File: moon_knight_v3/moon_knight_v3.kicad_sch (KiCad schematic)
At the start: 12 parts

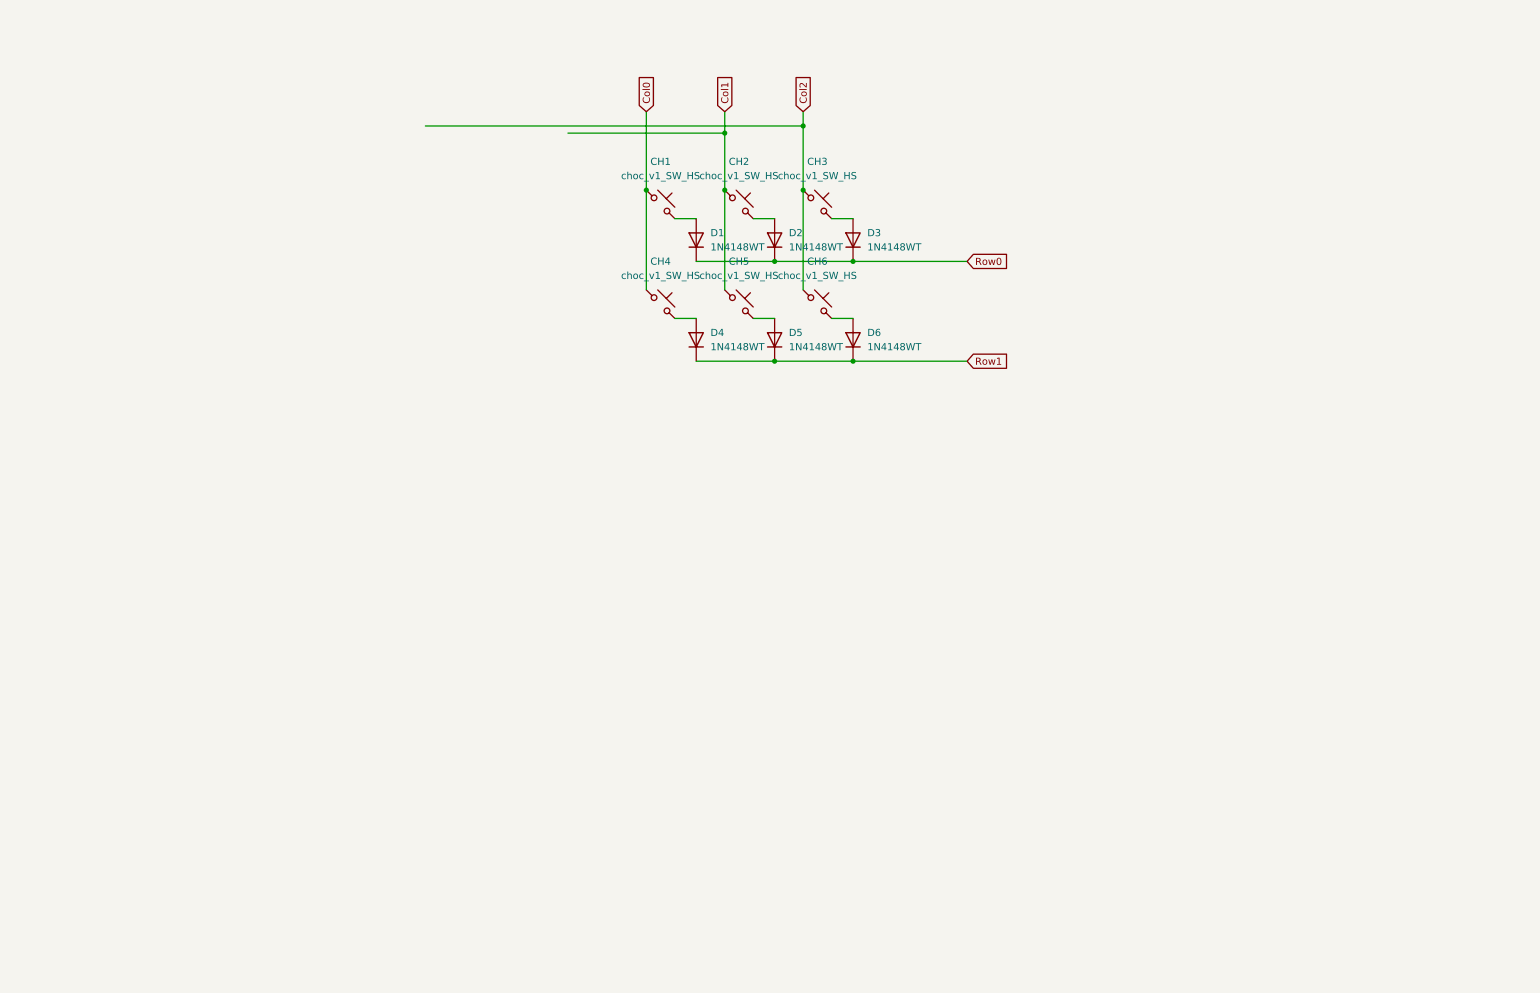
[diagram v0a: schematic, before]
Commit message: some commits
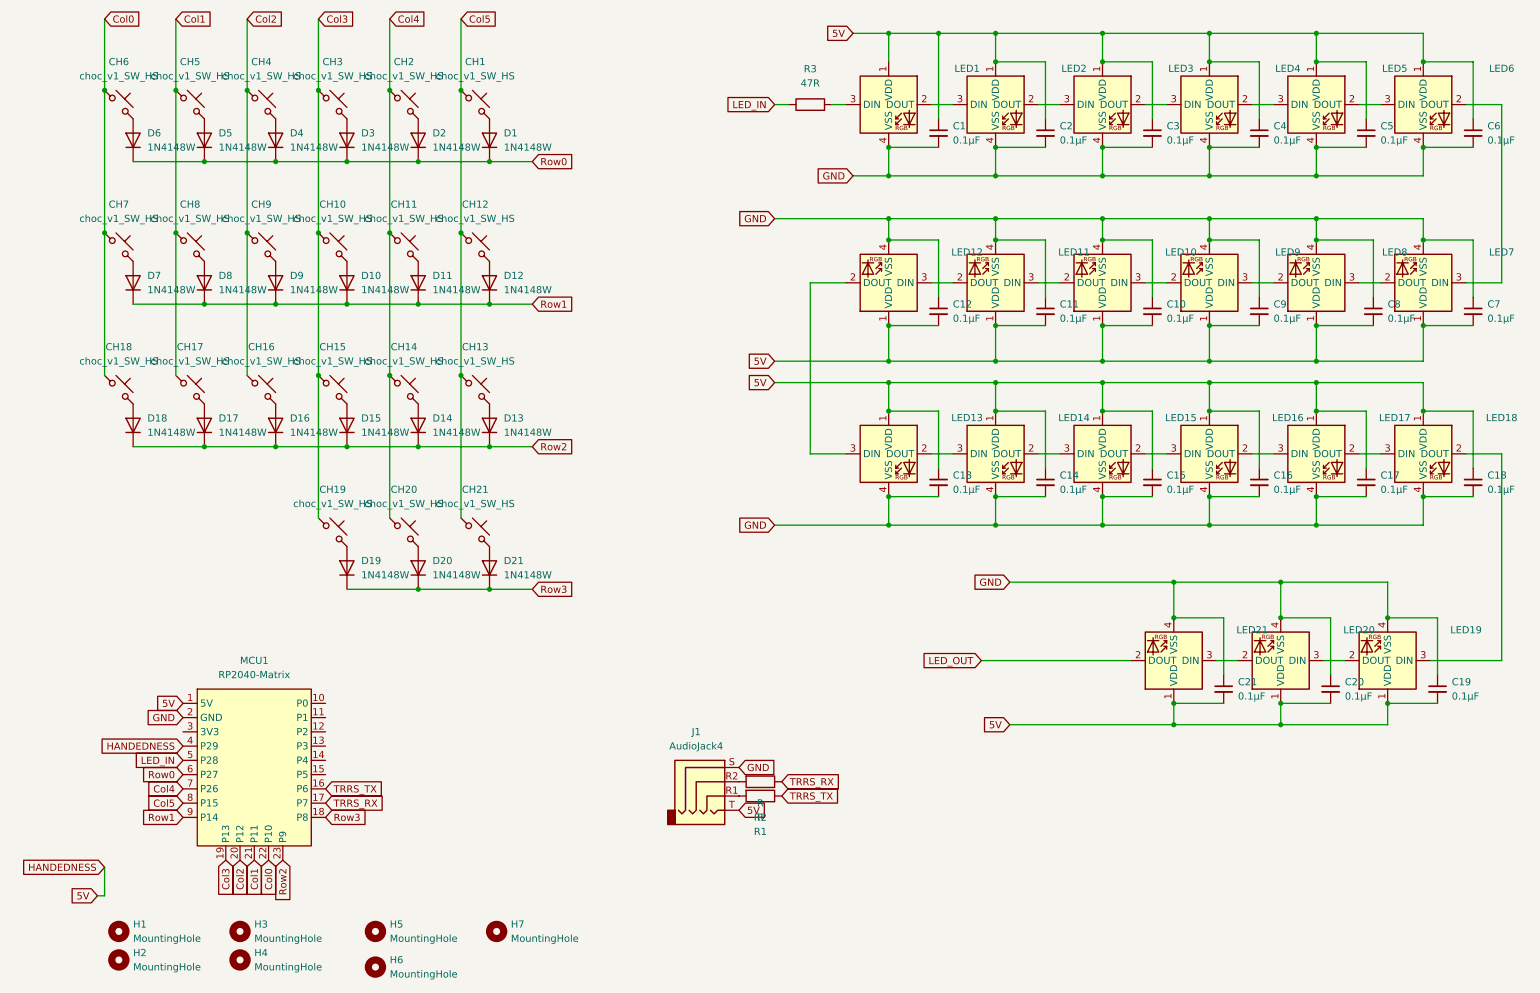
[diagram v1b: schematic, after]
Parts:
- removed D1, D2, D3, D4, D5, D6: 1N4148WT, Diode_SMD:D_SOD-523, symbol Diode:1N4148WT
- added C1, C10, C11, C12, C13, C14, C15, C16, C17, C18, C19, C2, C20, C21, C3, C4, C5, C6, C7, C8, C9: 0.1µF, Capacitor_SMD:C_1206_3216Metric, symbol Device:C_Small
- added CH10, CH11, CH12, CH13, CH14, CH15, CH16, CH17, CH18, CH19, CH20, CH7, CH8, CH9: choc_v1_SW_HS, PCM_marbastlib-choc:SW_choc_v1_HS_CPG135001S30_1u, symbol PCM_marbastlib-choc:choc_v1_SW_HS_CPG135001S30
- added CH21: choc_v1_SW_HS, PCM_marbastlib-choc:SW_choc_v1_HS_CPG135001S30_1.5u, symbol PCM_marbastlib-choc:choc_v1_SW_HS_CPG135001S30
- added D1, D10, D11, D12, D13, D14, D15, D16, D17, D18, D19, D2, D20, D21, D3, D4, D5, D6, D7, D8, D9: 1N4148W, ScottoKeebs_Components:Diode_SOD-123, symbol Diode:1N4148W
- added H1, H2, H3, H4, H5, H6, H7: MountingHole, MountingHole:MountingHole_2.2mm_M2, symbol Mechanical:MountingHole
- added J1: AudioJack4, PCM_marbastlib-xp-various:CON_MJ-4PP-9_Reversible, symbol Connector_Audio:AudioJack4
- added LED1, LED10, LED11, LED12, LED13, LED14, LED15, LED16, LED17, LED18, LED19, LED2, LED20, LED21, LED3, LED4, LED5, LED6, LED7, LED8, LED9: SK6812MINI-E, PCM_marbastlib-various:LED_6028R, symbol PCM_marbastlib-various:SK6812MINI-E
- added MCU1: RP2040-Matrix, PCM_marbastlib-xp-promicroish:RP2040-Matrix_AH, symbol PCM_marbastlib-promicroish:RP2040-Matrix
- added R1, R2: R, Resistor_SMD:R_1206_3216Metric_Pad1.30x1.75mm_HandSolder, symbol Device:R
- added R3: 47R, Resistor_SMD:R_1206_3216Metric_Pad1.30x1.75mm_HandSolder, symbol Device:R
- CH1: footprint key-switches:SW_MX_Kailh_Choc_V1V2_HotSwap_Hybrid_double -> PCM_marbastlib-choc:SW_choc_v1_HS_CPG135001S30_1u
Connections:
- net Col0: now also CH6.1, CH18.1, CH7.1, MCU1.22 (P10); no longer CH1.1, CH4.1
- net Col1: now also CH17.1, CH8.1, MCU1.21 (P11); no longer CH2.1
- net Col2: now also CH4.1, CH16.1, CH9.1, MCU1.20 (P12); no longer CH3.1, CH6.1
- net Row0: now also D1.1 (K), D2.1 (K), D3.1 (K), D4.1 (K), D5.1 (K), D6.1 (K), MCU1.6 (P27)
- net Row1: now also D10.1 (K), D11.1 (K), D12.1 (K), D7.1 (K), D8.1 (K), D9.1 (K), MCU1.9 (P14)
- net at CH6.2: now also D6.2 (A)
- net at CH4.2: now also D4.2 (A)
- net at CH3.2: now also D3.2 (A)
- net at CH2.2: now also D2.2 (A)
- net at CH5.2: now also D5.2 (A)
- net at CH1.2: now also D1.2 (A)
- new net: CH11.2, D11.2 (A)
- new net: CH14.2, D14.2 (A)
- new net: LED1.2 (DOUT), LED2.3 (DIN)
- new net: LED1.3 (DIN), R3.2
- new net: CH12.2, D12.2 (A)
- new net: CH15.2, D15.2 (A)
- new net: CH19.2, D19.2 (A)
- new net: CH7.2, D7.2 (A)
- new net: LED20.2 (DOUT), LED21.3 (DIN)
- new net: LED7.2 (DOUT), LED8.3 (DIN)
- new net: LED6.2 (DOUT), LED7.3 (DIN)
- new net: LED8.2 (DOUT), LED9.3 (DIN)
- new net: LED14.2 (DOUT), LED15.3 (DIN)
- new net: LED13.2 (DOUT), LED14.3 (DIN)
- new net: LED16.2 (DOUT), LED17.3 (DIN)
- new net: LED15.2 (DOUT), LED16.3 (DIN)
- new net: CH20.2, D20.2 (A)
- new net: LED17.2 (DOUT), LED18.3 (DIN)
- new net: CH13.2, D13.2 (A)
- new net: LED5.2 (DOUT), LED6.3 (DIN)
- new net: LED4.2 (DOUT), LED5.3 (DIN)
- new net: CH18.2, D18.2 (A)
- new net: CH16.2, D16.2 (A)
- new net: LED10.2 (DOUT), LED11.3 (DIN)
- new net: LED10.3 (DIN), LED9.2 (DOUT)
- new net: LED12.2 (DOUT), LED13.3 (DIN)
- new net: CH10.2, D10.2 (A)
- new net: LED19.2 (DOUT), LED20.3 (DIN)
- new net: CH9.2, D9.2 (A)
- new net: CH8.2, D8.2 (A)
- new net: CH21.2, D21.2 (A)
- new net: CH17.2, D17.2 (A)
- new net: LED11.2 (DOUT), LED12.3 (DIN)
- new net: LED2.2 (DOUT), LED3.3 (DIN)
- new net: LED18.2 (DOUT), LED19.3 (DIN)
- new net: LED3.2 (DOUT), LED4.3 (DIN)
- new net: J1.R2, R2.2
- new net: J1.R1, R1.2
- new net 5V: C1.1, C10.2, C11.2, C12.2, C13.1, C14.1, C15.1, C16.1, C17.1, C18.1, C19.2, C2.1, C20.2, C21.2, C3.1, C4.1, C5.1, C6.1, C7.2, C8.2, C9.2, J1.T, LED1.1 (VDD), LED10.1 (VDD), LED11.1 (VDD), LED12.1 (VDD), LED13.1 (VDD), LED14.1 (VDD), LED15.1 (VDD), LED16.1 (VDD), LED17.1 (VDD), LED18.1 (VDD), LED19.1 (VDD), LED2.1 (VDD), LED20.1 (VDD), LED21.1 (VDD), LED3.1 (VDD), LED4.1 (VDD), LED5.1 (VDD), LED6.1 (VDD), LED7.1 (VDD), LED8.1 (VDD), LED9.1 (VDD), MCU1.1 (5V), MCU1.4 (P29)
- new net Col3: CH10.1, CH15.1, CH19.1, CH3.1, MCU1.19 (P13)
- new net Col4: CH11.1, CH14.1, CH2.1, CH20.1, MCU1.7 (P26)
- new net Col5: CH1.1, CH12.1, CH13.1, CH21.1, MCU1.8 (P15)
- new net GND: C1.2, C10.1, C11.1, C12.1, C13.2, C14.2, C15.2, C16.2, C17.2, C18.2, C19.1, C2.2, C20.1, C21.1, C3.2, C4.2, C5.2, C6.2, C7.1, C8.1, C9.1, J1.S, LED1.4 (VSS), LED10.4 (VSS), LED11.4 (VSS), LED12.4 (VSS), LED13.4 (VSS), LED14.4 (VSS), LED15.4 (VSS), LED16.4 (VSS), LED17.4 (VSS), LED18.4 (VSS), LED19.4 (VSS), LED2.4 (VSS), LED20.4 (VSS), LED21.4 (VSS), LED3.4 (VSS), LED4.4 (VSS), LED5.4 (VSS), LED6.4 (VSS), LED7.4 (VSS), LED8.4 (VSS), LED9.4 (VSS), MCU1.2 (GND)
- new net LED_IN: MCU1.5 (P28), R3.1
- new net LED_OUT: LED21.2 (DOUT)
- new net Row2: D13.1 (K), D14.1 (K), D15.1 (K), D16.1 (K), D17.1 (K), D18.1 (K), MCU1.23 (P9)
- new net Row3: D19.1 (K), D20.1 (K), D21.1 (K), MCU1.18 (P8)
- new net TRRS_RX: MCU1.17 (P7), R2.1
- new net TRRS_TX: MCU1.16 (P6), R1.1
